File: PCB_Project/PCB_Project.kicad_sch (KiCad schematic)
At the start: 1 part

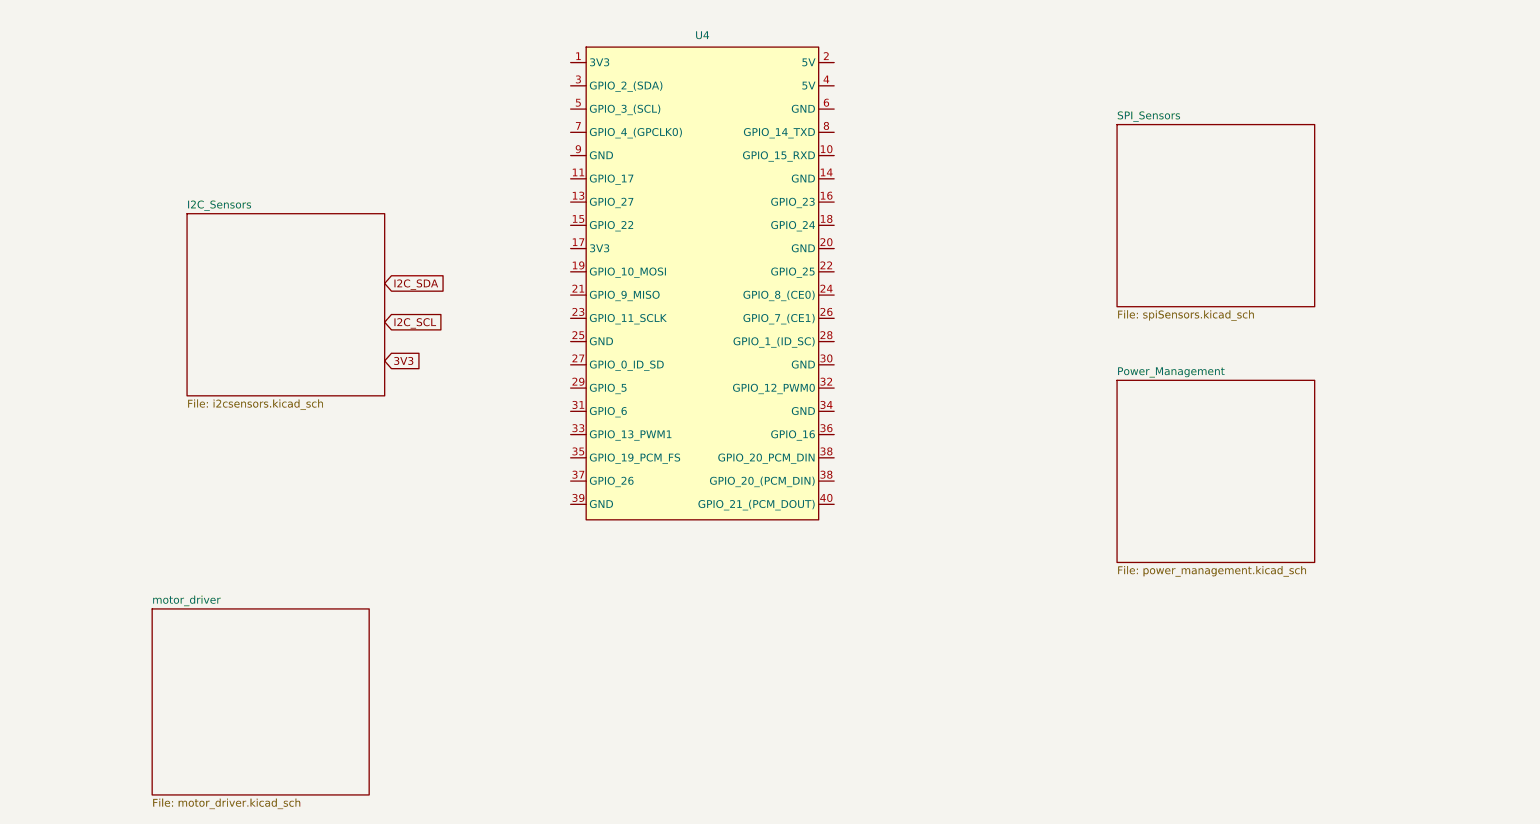
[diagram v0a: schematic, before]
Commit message: ignore how ugly it looks I need to fix it
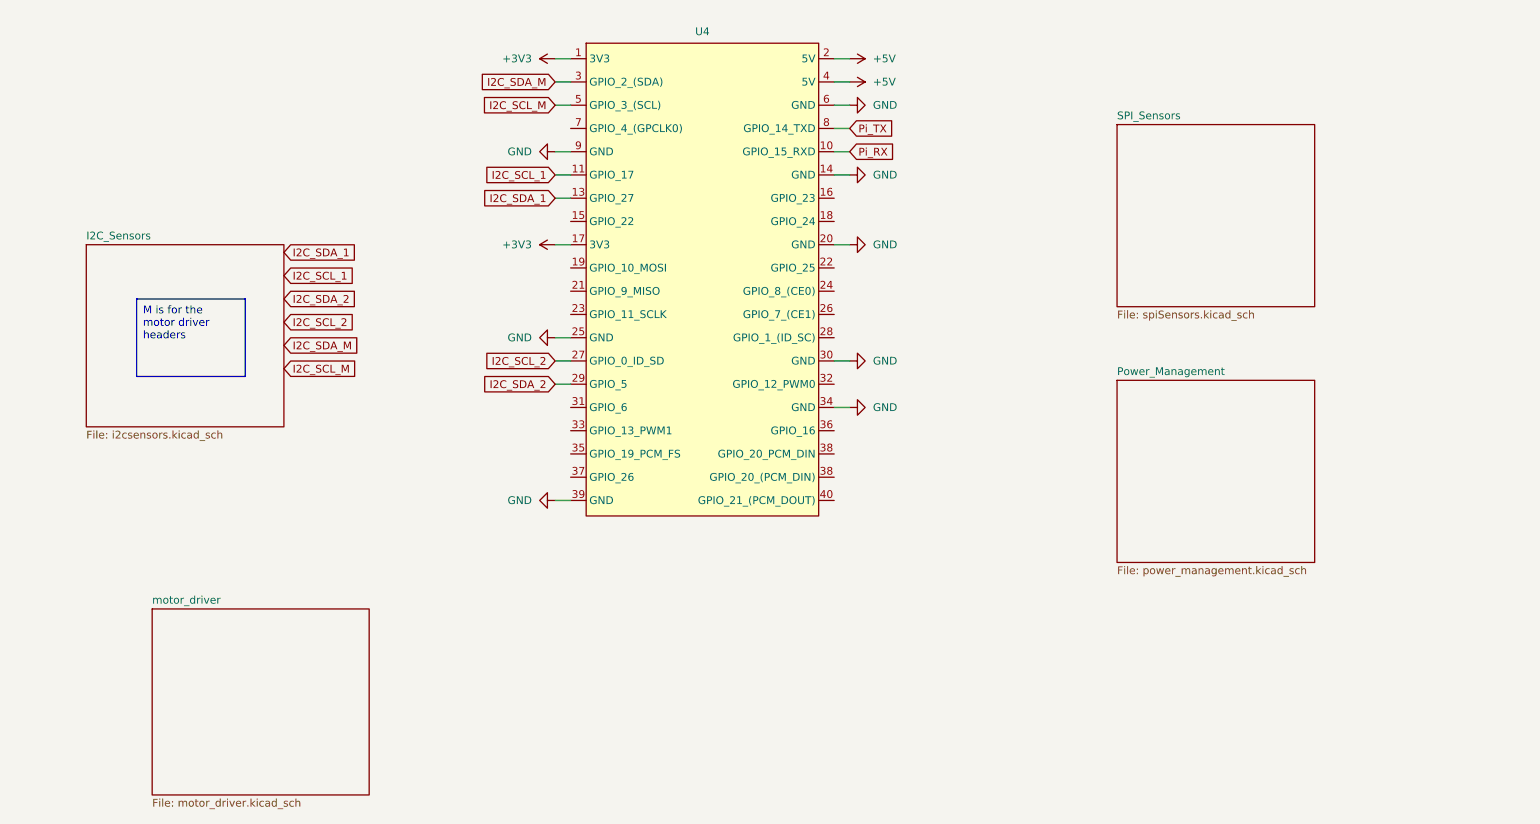
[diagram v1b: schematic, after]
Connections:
- net +3V3: now reaches U4.1 (3V3)
- net +3V3: now also U4.17 (3V3)
- net Pi_RX: now reaches U4.10 (GPIO_15_RXD)
- net I2C_SCL_1: now reaches U4.11 (GPIO_17)
- net I2C_SDA_1: now reaches U4.13 (GPIO_27)
- net GND: now reaches U4.14 (GND)
- net GND: now also U4.20 (GND), U4.25 (GND), U4.30 (GND), U4.34 (GND), U4.39 (GND), U4.6 (GND), U4.9 (GND)
- net +5V: now reaches U4.2 (5V)
- net +5V: now also U4.4 (5V)
- net I2C_SCL_2: now reaches U4.27 (GPIO_0_ID_SD)
- net I2C_SDA_2: now reaches U4.29 (GPIO_5)
- net I2C_SDA_M: now reaches U4.3 (GPIO_2_(SDA))
- net I2C_SCL_M: now reaches U4.5 (GPIO_3_(SCL))
- net Pi_TX: now reaches U4.8 (GPIO_14_TXD)
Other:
- moved on the sheet: U4

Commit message: work baby
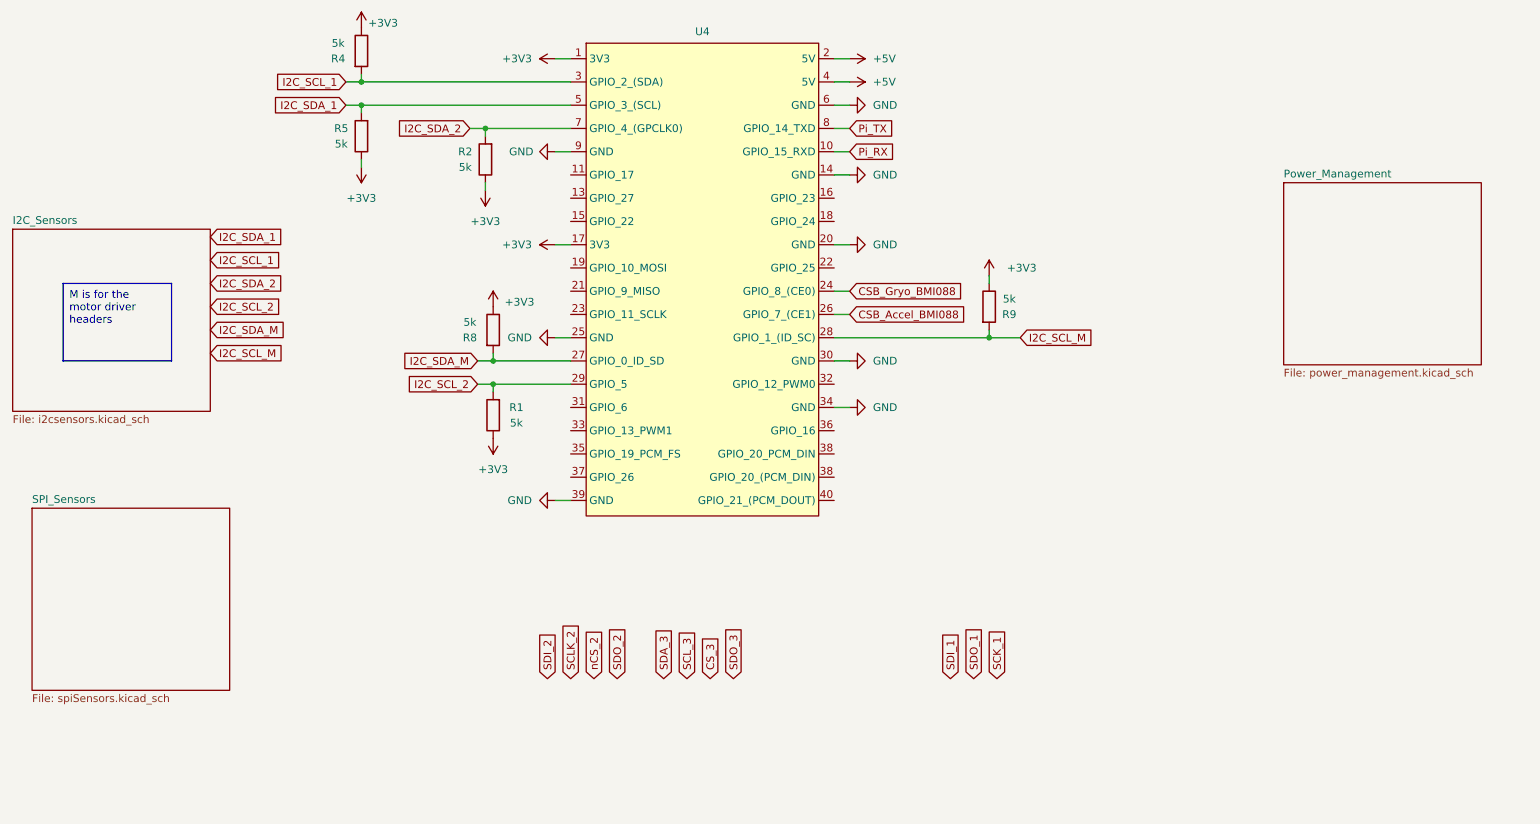
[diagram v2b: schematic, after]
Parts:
- added R1, R2, R4, R5, R8, R9: 5k, Resistor_SMD:R_0603_1608Metric, symbol Device:R
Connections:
- net +3V3: now also R1.1, R2.1, R4.1, R5.1, R8.1, R9.1
- net I2C_SCL_1: now also U4.3 (GPIO_2_(SDA)), R4.2; no longer U4.11 (GPIO_17)
- net I2C_SCL_2: now also U4.29 (GPIO_5), R1.2; no longer U4.27 (GPIO_0_ID_SD)
- net I2C_SCL_M: now also U4.28 (GPIO_1_(ID_SC)), R9.2; no longer U4.5 (GPIO_3_(SCL))
- net I2C_SDA_1: now also U4.5 (GPIO_3_(SCL)), R5.2; no longer U4.13 (GPIO_27)
- net I2C_SDA_2: now also U4.7 (GPIO_4_(GPCLK0)), R2.2; no longer U4.29 (GPIO_5)
- net I2C_SDA_M: now also U4.27 (GPIO_0_ID_SD), R8.2; no longer U4.3 (GPIO_2_(SDA))
- net CSB_Gryo_BMI088: now reaches U4.24 (GPIO_8_(CE0))
- net CSB_Accel_BMI088: now reaches U4.26 (GPIO_7_(CE1))
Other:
- removed sheet motor_driver
